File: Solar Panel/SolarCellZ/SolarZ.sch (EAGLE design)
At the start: 34 parts, among them X1 BU-SMA-V

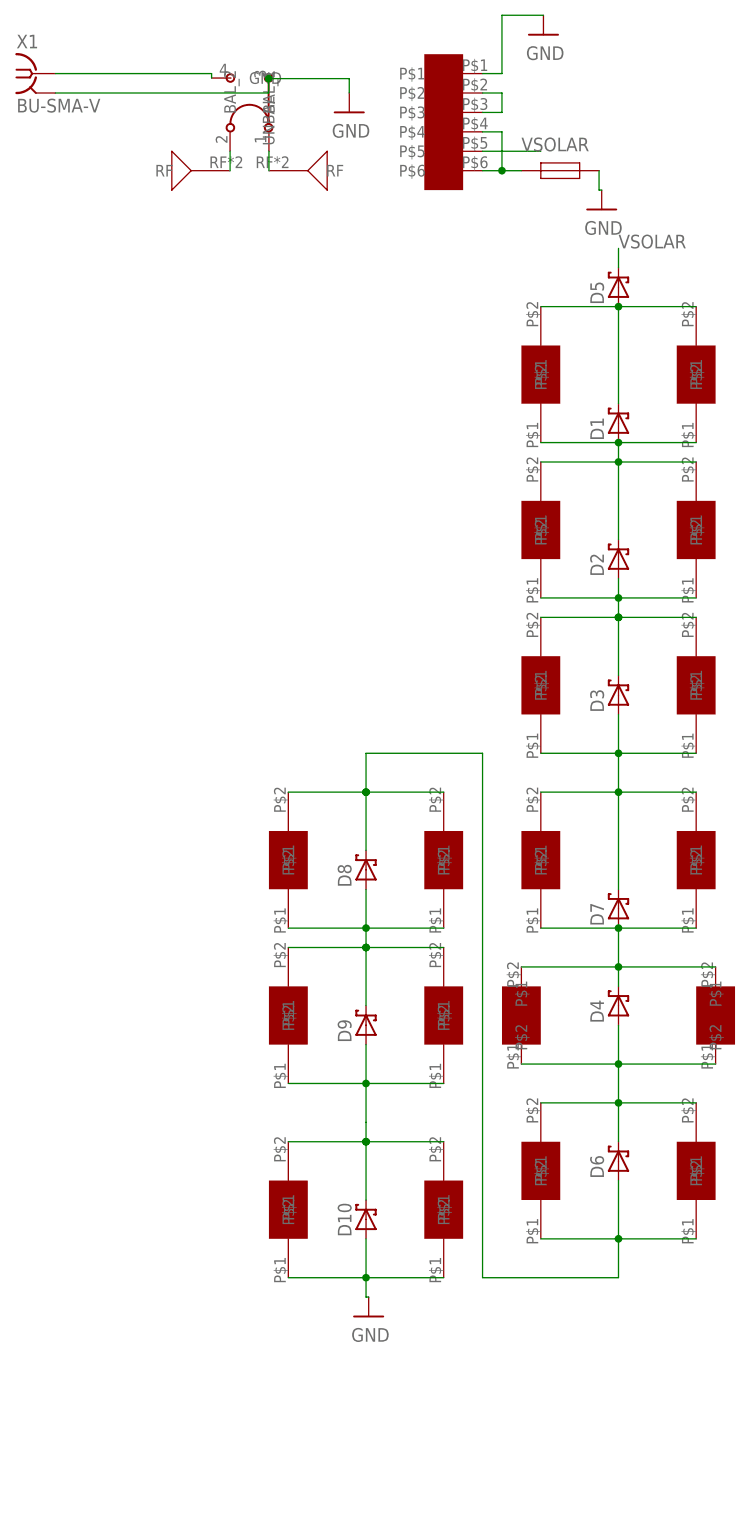
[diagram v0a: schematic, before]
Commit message: Magnetorquers done
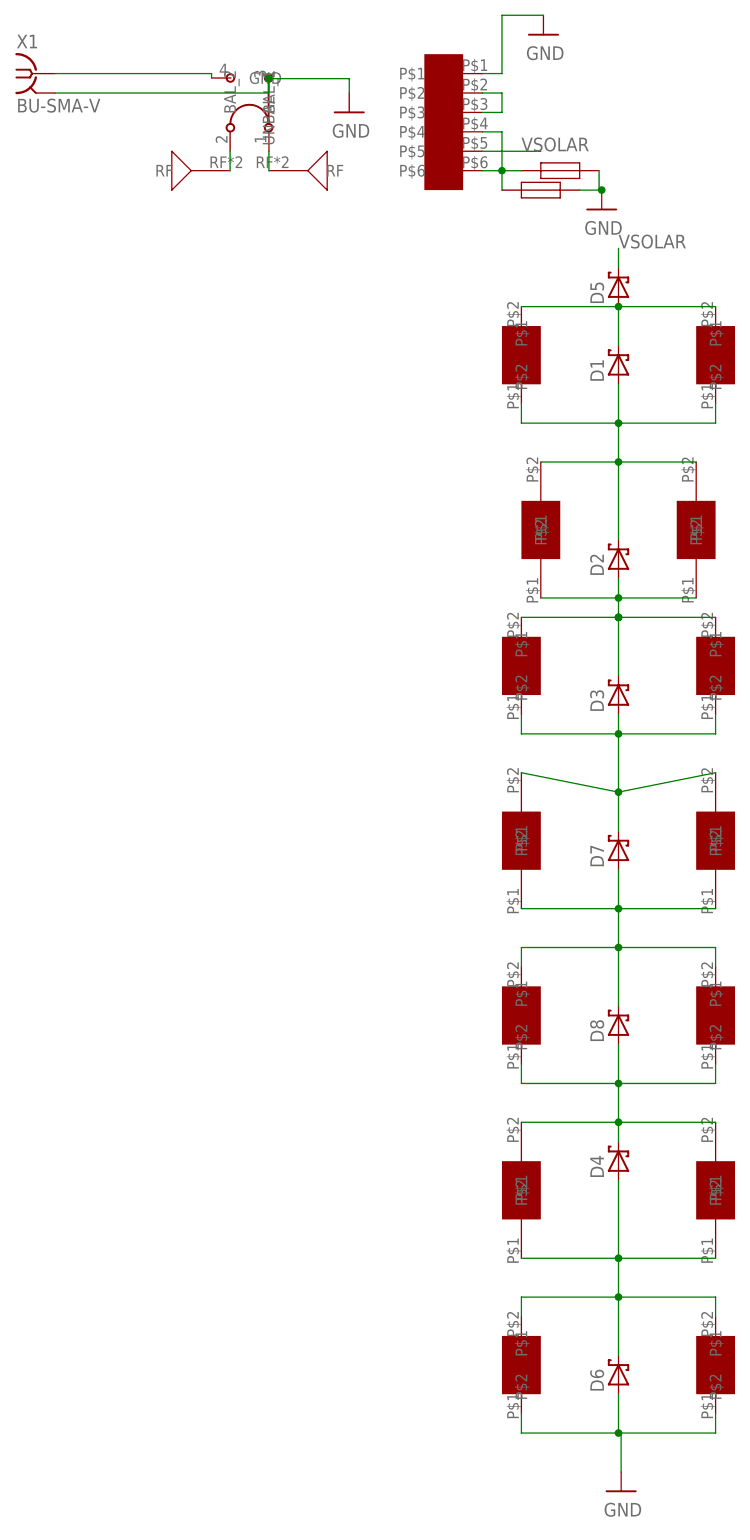
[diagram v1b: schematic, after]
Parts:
- removed 15, 16, 17, 18: KXOB22-04X3F, Solar:KXOB22-04X3F
- removed D10, D9: SB_DIODE, Solar:SB_DIODE
- added F1: (no value), pandasat:BURN_TERM
- 12, 14, 2, 3, 4, 5, 8, 9: value KXOB22-04X3F -> SLMD121H04L; device Solar:KXOB22-04X3F -> Solar:SLMD121H04L
- 6, 7: value SLMD121H04L -> KXOB22-04X3F; device Solar:SLMD121H04L -> Solar:KXOB22-04X3F
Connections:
- removed net N$14: 12.P$1, 14.P$1, 15.P$2, 16.P$2, D8.POS, D9.NEG
- removed net N$18: 12.P$2, 14.P$2, 8.P$1, 9.P$1, D6.POS, D8.NEG
- removed net N$4: U$1.BAL_1, U$3.RF
- new net N8: 12.P$1, 14.P$1, 6.P$2, 7.P$2, D4.NEG, D8.POS
- net GND: now also 8.P$1, 9.P$1, D6.POS, F1.2; no longer 17.P$1, 18.P$1, D10.POS
- net N$1: now also U$1.BAL_2, U$3.RF; no longer 15.P$1, 16.P$1, 17.P$2, 18.P$2, D10.NEG, D9.POS
- net N$16: now also F1.1
- net N$3: now also U$1.BAL_1; no longer U$1.BAL_2
- net N$9: now also 12.P$2, 14.P$2, D8.NEG; no longer 6.P$2, 7.P$2, D4.NEG
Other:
- moved on the sheet: D1, D4, D6, D7, D8
